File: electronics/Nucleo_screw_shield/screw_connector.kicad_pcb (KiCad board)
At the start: 2 copper layers, 91 x 101.3 mm, 360 parts, among them J1 Conn_01x03, J10 Conn_01x06, J11 Conn_01x10, J12 Conn_01x08, J13 Conn_01x03, J14 Conn_01x03, J15 Conn_01x03, J16 Conn_01x03, J17 Conn_01x03, J18 Conn_01x02, J19 Conn_01x03, J2 Conn_02x19_Odd_Even, J20 Conn_01x03, J21 Conn_01x03, J22 Conn_01x03, J23 Conn_01x03, J3 Conn_01x08, J4 Conn_01x06, J5 Conn_01x10, J6 Conn_01x08, J7 Conn_02x19_Odd_Even, J8 Conn_01x03, J9 Conn_01x08

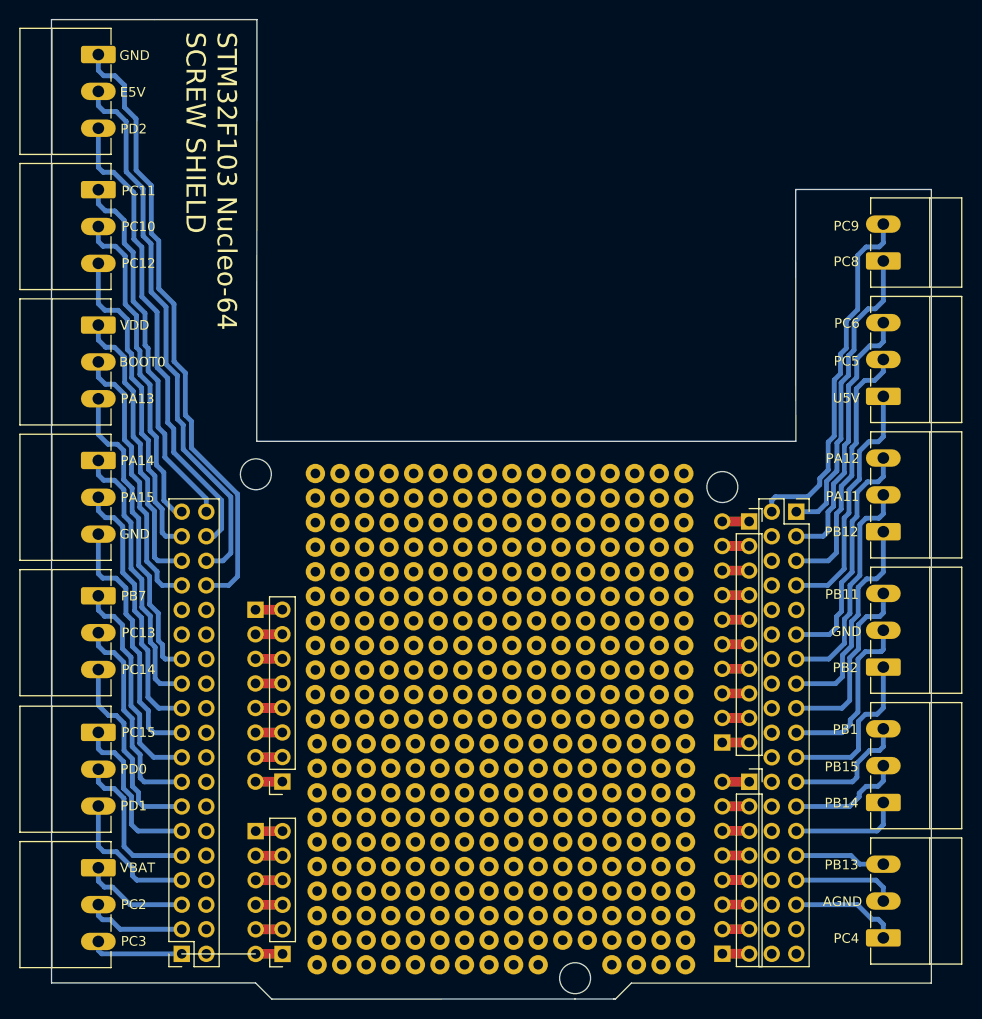
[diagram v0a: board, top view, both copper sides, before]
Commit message: Reorganize CAD files
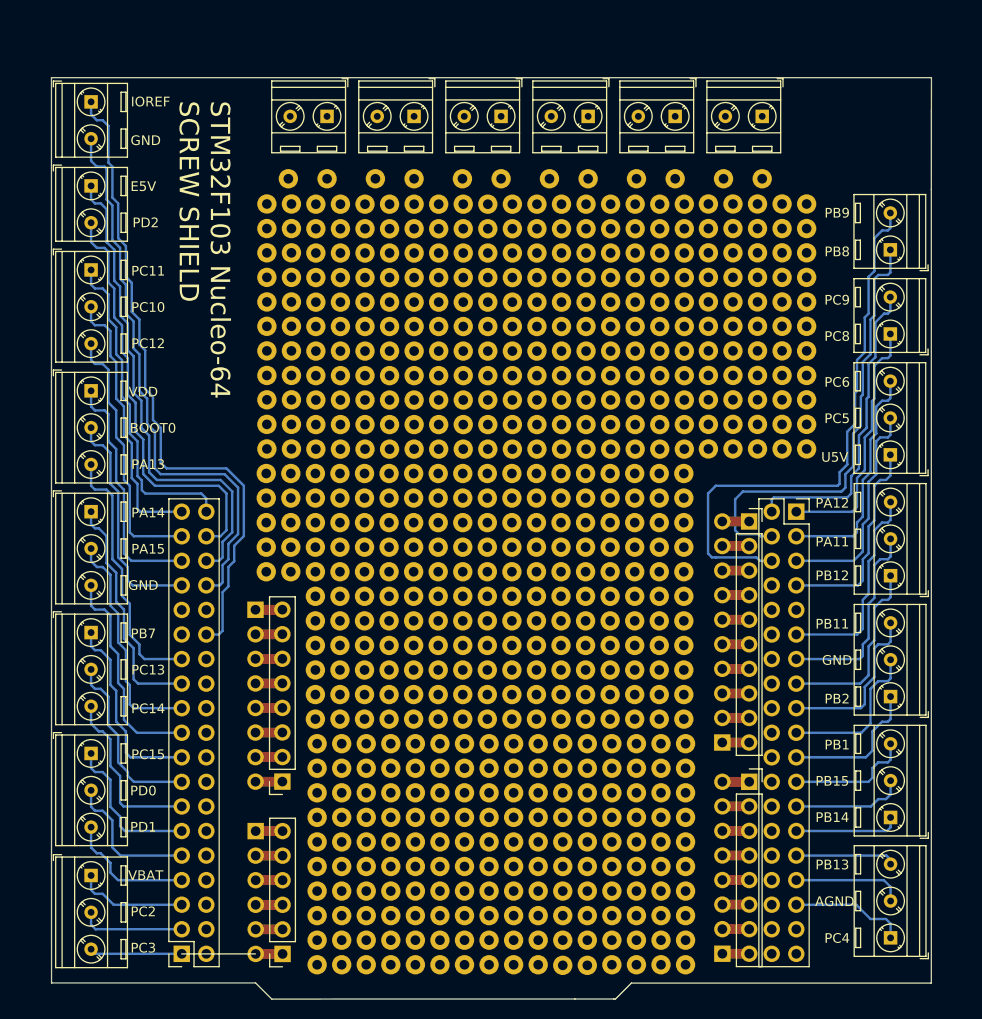
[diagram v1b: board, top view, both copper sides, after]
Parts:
- removed the REF** at (164.7, 146.1)
- removed the REF** at (179.9, 95.3)
- removed the REF** at (131.6, 94.0)
- added J24: Conn_01x02, TerminalBlock_MetzConnect:TerminalBlock_MetzConnect_Type086_RT03402HBLC_1x02_P3.81mm_Horizontal, F.Cu at (114.6, 64.2)
- added J25: Conn_01x02, TerminalBlock_MetzConnect:TerminalBlock_MetzConnect_Type086_RT03402HBLC_1x02_P3.81mm_Horizontal, F.Cu at (197.2, 70.8)
- added J26: Conn_01x02, TerminalBlock_MetzConnect:TerminalBlock_MetzConnect_Type086_RT03402HBLC_1x02_P3.81mm_Horizontal, F.Cu at (184.0, 57.0)
- added J27: Conn_01x02, TerminalBlock_MetzConnect:TerminalBlock_MetzConnect_Type086_RT03402HBLC_1x02_P3.81mm_Horizontal, F.Cu at (139.0, 57.0)
- added J28: Conn_01x02, TerminalBlock_MetzConnect:TerminalBlock_MetzConnect_Type086_RT03402HBLC_1x02_P3.81mm_Horizontal, F.Cu at (175.0, 57.0)
- added J29: Conn_01x02, TerminalBlock_MetzConnect:TerminalBlock_MetzConnect_Type086_RT03402HBLC_1x02_P3.81mm_Horizontal, F.Cu at (148.0, 57.0)
- added J30: Conn_01x02, TerminalBlock_MetzConnect:TerminalBlock_MetzConnect_Type086_RT03402HBLC_1x02_P3.81mm_Horizontal, F.Cu at (166.0, 57.0)
- added J31: Conn_01x02, TerminalBlock_MetzConnect:TerminalBlock_MetzConnect_Type086_RT03402HBLC_1x02_P3.81mm_Horizontal, F.Cu at (157.0, 57.0)
- added REF**: hole 1mm, Connector_PinHeader_2.54mm:hole 1mm, F.Cu at (186.1, 66.1)
- added REF**: hole 1mm, Connector_PinHeader_2.54mm:hole 1mm, F.Cu at (181.0, 66.1)
- added REF**: hole 1mm, Connector_PinHeader_2.54mm:hole 1mm, F.Cu at (137.8, 68.7)
- added REF**: hole 1mm, Connector_PinHeader_2.54mm:hole 1mm, F.Cu at (175.9, 66.1)
- added REF**: hole 1mm, Connector_PinHeader_2.54mm:hole 1mm, F.Cu at (163.2, 66.1)
- added REF**: hole 1mm, Connector_PinHeader_2.54mm:hole 1mm, F.Cu at (160.7, 66.1)
- added REF**: hole 1mm, Connector_PinHeader_2.54mm:hole 1mm, F.Cu at (158.2, 68.7)
- added REF**: hole 1mm, Connector_PinHeader_2.54mm:hole 1mm, F.Cu at (145.5, 68.7)
- added REF**: hole 1mm, Connector_PinHeader_2.54mm:hole 1mm, F.Cu at (150.5, 68.7)
- added REF**: hole 1mm, Connector_PinHeader_2.54mm:hole 1mm, F.Cu at (155.6, 68.7)
- added REF**: hole 1mm, Connector_PinHeader_2.54mm:hole 1mm, F.Cu at (142.9, 66.1)
- added REF**: hole 1mm, Connector_PinHeader_2.54mm:hole 1mm, F.Cu at (148.0, 66.1)
- added REF**: hole 1mm, Connector_PinHeader_2.54mm:hole 1mm, F.Cu at (178.4, 88.9)
- added REF**: hole 1mm, Connector_PinHeader_2.54mm:hole 1mm, F.Cu at (140.4, 68.7)
- added REF**: hole 1mm, Connector_PinHeader_2.54mm:hole 1mm, F.Cu at (155.6, 66.1)
- added REF**: hole 1mm, Connector_PinHeader_2.54mm:hole 1mm, F.Cu at (142.9, 68.7)
- added REF**: hole 1mm, Connector_PinHeader_2.54mm:hole 1mm, F.Cu at (173.4, 68.7)
- added REF**: hole 1mm, Connector_PinHeader_2.54mm:hole 1mm, F.Cu at (170.9, 66.1)
- added REF**: hole 1mm, Connector_PinHeader_2.54mm:hole 1mm, F.Cu at (168.3, 66.1)
- added REF**: hole 1mm, Connector_PinHeader_2.54mm:hole 1mm, F.Cu at (158.2, 66.1)
- added REF**: hole 1mm, Connector_PinHeader_2.54mm:hole 1mm, F.Cu at (170.9, 68.7)
- added REF**: hole 1mm, Connector_PinHeader_2.54mm:hole 1mm, F.Cu at (163.2, 68.7)
- added REF**: hole 1mm, Connector_PinHeader_2.54mm:hole 1mm, F.Cu at (165.8, 68.7)
- added REF**: hole 1mm, Connector_PinHeader_2.54mm:hole 1mm, F.Cu at (186.1, 91.4)
- added REF**: hole 1mm, Connector_PinHeader_2.54mm:hole 1mm, F.Cu at (165.9, 144.8)
- added REF**: hole 1mm, Connector_PinHeader_2.54mm:hole 1mm, F.Cu at (163.4, 144.8)
- added REF**: hole 1mm, Connector_PinHeader_2.54mm:hole 1mm, F.Cu at (148.0, 76.3)
- added REF**: hole 1mm, Connector_PinHeader_2.54mm:hole 1mm, F.Cu at (145.5, 76.3)
- added REF**: hole 1mm, Connector_PinHeader_2.54mm:hole 1mm, F.Cu at (150.5, 76.3)
- added REF**: hole 1mm, Connector_PinHeader_2.54mm:hole 1mm, F.Cu at (153.1, 76.3)
- added REF**: hole 1mm, Connector_PinHeader_2.54mm:hole 1mm, F.Cu at (140.4, 76.3)
- added REF**: hole 1mm, Connector_PinHeader_2.54mm:hole 1mm, F.Cu at (142.9, 76.3)
- added REF**: hole 1mm, Connector_PinHeader_2.54mm:hole 1mm, F.Cu at (137.8, 76.3)
- added REF**: hole 1mm, Connector_PinHeader_2.54mm:hole 1mm, F.Cu at (153.1, 71.2)
- added REF**: hole 1mm, Connector_PinHeader_2.54mm:hole 1mm, F.Cu at (178.4, 91.4)
- added REF**: hole 1mm, Connector_PinHeader_2.54mm:hole 1mm, F.Cu at (145.5, 71.2)
- added REF**: hole 1mm, Connector_PinHeader_2.54mm:hole 1mm, F.Cu at (137.8, 71.2)
- added REF**: hole 1mm, Connector_PinHeader_2.54mm:hole 1mm, F.Cu at (173.4, 71.2)
- added REF**: hole 1mm, Connector_PinHeader_2.54mm:hole 1mm, F.Cu at (140.4, 71.2)
- added REF**: hole 1mm, Connector_PinHeader_2.54mm:hole 1mm, F.Cu at (158.2, 71.2)
- added REF**: hole 1mm, Connector_PinHeader_2.54mm:hole 1mm, F.Cu at (170.9, 73.7)
- added REF**: hole 1mm, Connector_PinHeader_2.54mm:hole 1mm, F.Cu at (142.9, 73.7)
- added REF**: hole 1mm, Connector_PinHeader_2.54mm:hole 1mm, F.Cu at (168.3, 71.2)
- added REF**: hole 1mm, Connector_PinHeader_2.54mm:hole 1mm, F.Cu at (170.9, 71.2)
- added REF**: hole 1mm, Connector_PinHeader_2.54mm:hole 1mm, F.Cu at (173.4, 73.7)
- added REF**: hole 1mm, Connector_PinHeader_2.54mm:hole 1mm, F.Cu at (188.6, 88.9)
- added REF**: hole 1mm, Connector_PinHeader_2.54mm:hole 1mm, F.Cu at (155.6, 73.7)
- added REF**: hole 1mm, Connector_PinHeader_2.54mm:hole 1mm, F.Cu at (155.6, 71.2)
- added REF**: hole 1mm, Connector_PinHeader_2.54mm:hole 1mm, F.Cu at (140.4, 73.7)
- added REF**: hole 1mm, Connector_PinHeader_2.54mm:hole 1mm, F.Cu at (148.0, 71.2)
- added REF**: hole 1mm, Connector_PinHeader_2.54mm:hole 1mm, F.Cu at (142.9, 71.2)
- added REF**: hole 1mm, Connector_PinHeader_2.54mm:hole 1mm, F.Cu at (150.5, 73.7)
- added REF**: hole 1mm, Connector_PinHeader_2.54mm:hole 1mm, F.Cu at (163.2, 73.7)
- added REF**: hole 1mm, Connector_PinHeader_2.54mm:hole 1mm, F.Cu at (160.7, 76.3)
- added REF**: hole 1mm, Connector_PinHeader_2.54mm:hole 1mm, F.Cu at (163.2, 76.3)
- added REF**: hole 1mm, Connector_PinHeader_2.54mm:hole 1mm, F.Cu at (155.6, 76.3)
- added REF**: hole 1mm, Connector_PinHeader_2.54mm:hole 1mm, F.Cu at (181.0, 88.9)
- added REF**: hole 1mm, Connector_PinHeader_2.54mm:hole 1mm, F.Cu at (158.2, 76.3)
- added REF**: hole 1mm, Connector_PinHeader_2.54mm:hole 1mm, F.Cu at (165.8, 73.7)
- added REF**: hole 1mm, Connector_PinHeader_2.54mm:hole 1mm, F.Cu at (158.2, 73.7)
- added REF**: hole 1mm, Connector_PinHeader_2.54mm:hole 1mm, F.Cu at (153.1, 73.7)
- added REF**: hole 1mm, Connector_PinHeader_2.54mm:hole 1mm, F.Cu at (145.5, 73.7)
- added REF**: hole 1mm, Connector_PinHeader_2.54mm:hole 1mm, F.Cu at (148.0, 73.7)
- added REF**: hole 1mm, Connector_PinHeader_2.54mm:hole 1mm, F.Cu at (160.7, 73.7)
- added REF**: hole 1mm, Connector_PinHeader_2.54mm:hole 1mm, F.Cu at (173.4, 76.3)
- added REF**: hole 1mm, Connector_PinHeader_2.54mm:hole 1mm, F.Cu at (168.3, 73.7)
- added REF**: hole 1mm, Connector_PinHeader_2.54mm:hole 1mm, F.Cu at (137.8, 73.7)
- added REF**: hole 1mm, Connector_PinHeader_2.54mm:hole 1mm, F.Cu at (183.5, 91.4)
- added REF**: hole 1mm, Connector_PinHeader_2.54mm:hole 1mm, F.Cu at (168.3, 76.3)
- added REF**: hole 1mm, Connector_PinHeader_2.54mm:hole 1mm, F.Cu at (170.9, 76.3)
- added REF**: hole 1mm, Connector_PinHeader_2.54mm:hole 1mm, F.Cu at (175.9, 73.7)
- added REF**: hole 1mm, Connector_PinHeader_2.54mm:hole 1mm, F.Cu at (165.8, 76.3)
- added REF**: hole 1mm, Connector_PinHeader_2.54mm:hole 1mm, F.Cu at (150.5, 71.2)
- added REF**: hole 1mm, Connector_PinHeader_2.54mm:hole 1mm, F.Cu at (160.7, 71.2)
- added REF**: hole 1mm, Connector_PinHeader_2.54mm:hole 1mm, F.Cu at (165.8, 71.2)
- added REF**: hole 1mm, Connector_PinHeader_2.54mm:hole 1mm, F.Cu at (163.2, 71.2)
- added REF**: hole 1mm, Connector_PinHeader_2.54mm:hole 1mm, F.Cu at (175.9, 71.2)
- added REF**: hole 1mm, Connector_PinHeader_2.54mm:hole 1mm, F.Cu at (175.9, 76.3)
- added REF**: hole 1mm, Connector_PinHeader_2.54mm:hole 1mm, F.Cu at (181.0, 91.4)
- added REF**: hole 1mm, Connector_PinHeader_2.54mm:hole 1mm, F.Cu at (148.0, 83.9)
- added REF**: hole 1mm, Connector_PinHeader_2.54mm:hole 1mm, F.Cu at (145.5, 83.9)
- added REF**: hole 1mm, Connector_PinHeader_2.54mm:hole 1mm, F.Cu at (150.5, 83.9)
- added REF**: hole 1mm, Connector_PinHeader_2.54mm:hole 1mm, F.Cu at (153.1, 83.9)
- added REF**: hole 1mm, Connector_PinHeader_2.54mm:hole 1mm, F.Cu at (140.4, 83.9)
- added REF**: hole 1mm, Connector_PinHeader_2.54mm:hole 1mm, F.Cu at (142.9, 83.9)
- added REF**: hole 1mm, Connector_PinHeader_2.54mm:hole 1mm, F.Cu at (137.8, 83.9)
- added REF**: hole 1mm, Connector_PinHeader_2.54mm:hole 1mm, F.Cu at (153.1, 78.8)
- added REF**: hole 1mm, Connector_PinHeader_2.54mm:hole 1mm, F.Cu at (145.5, 78.8)
- added REF**: hole 1mm, Connector_PinHeader_2.54mm:hole 1mm, F.Cu at (137.8, 78.8)
- added REF**: hole 1mm, Connector_PinHeader_2.54mm:hole 1mm, F.Cu at (183.5, 86.4)
- added REF**: hole 1mm, Connector_PinHeader_2.54mm:hole 1mm, F.Cu at (173.4, 78.8)
- added REF**: hole 1mm, Connector_PinHeader_2.54mm:hole 1mm, F.Cu at (140.4, 78.8)
- added REF**: hole 1mm, Connector_PinHeader_2.54mm:hole 1mm, F.Cu at (158.2, 78.8)
- added REF**: hole 1mm, Connector_PinHeader_2.54mm:hole 1mm, F.Cu at (170.9, 81.3)
- added REF**: hole 1mm, Connector_PinHeader_2.54mm:hole 1mm, F.Cu at (142.9, 81.3)
- added REF**: hole 1mm, Connector_PinHeader_2.54mm:hole 1mm, F.Cu at (168.3, 78.8)
- added REF**: hole 1mm, Connector_PinHeader_2.54mm:hole 1mm, F.Cu at (170.9, 78.8)
- added REF**: hole 1mm, Connector_PinHeader_2.54mm:hole 1mm, F.Cu at (173.4, 81.3)
- added REF**: hole 1mm, Connector_PinHeader_2.54mm:hole 1mm, F.Cu at (155.6, 81.3)
- added REF**: hole 1mm, Connector_PinHeader_2.54mm:hole 1mm, F.Cu at (155.6, 78.8)
- added REF**: hole 1mm, Connector_PinHeader_2.54mm:hole 1mm, F.Cu at (183.5, 88.9)
- added REF**: hole 1mm, Connector_PinHeader_2.54mm:hole 1mm, F.Cu at (140.4, 81.3)
- added REF**: hole 1mm, Connector_PinHeader_2.54mm:hole 1mm, F.Cu at (148.0, 78.8)
- added REF**: hole 1mm, Connector_PinHeader_2.54mm:hole 1mm, F.Cu at (142.9, 78.8)
- added REF**: hole 1mm, Connector_PinHeader_2.54mm:hole 1mm, F.Cu at (150.5, 81.3)
- added REF**: hole 1mm, Connector_PinHeader_2.54mm:hole 1mm, F.Cu at (163.2, 81.3)
- added REF**: hole 1mm, Connector_PinHeader_2.54mm:hole 1mm, F.Cu at (160.7, 83.9)
- added REF**: hole 1mm, Connector_PinHeader_2.54mm:hole 1mm, F.Cu at (163.2, 83.9)
- added REF**: hole 1mm, Connector_PinHeader_2.54mm:hole 1mm, F.Cu at (155.6, 83.9)
- added REF**: hole 1mm, Connector_PinHeader_2.54mm:hole 1mm, F.Cu at (158.2, 83.9)
- added REF**: hole 1mm, Connector_PinHeader_2.54mm:hole 1mm, F.Cu at (165.8, 81.3)
- added REF**: hole 1mm, Connector_PinHeader_2.54mm:hole 1mm, F.Cu at (178.4, 66.1)
- added REF**: hole 1mm, Connector_PinHeader_2.54mm:hole 1mm, F.Cu at (186.1, 88.9)
- added REF**: hole 1mm, Connector_PinHeader_2.54mm:hole 1mm, F.Cu at (158.2, 81.3)
- added REF**: hole 1mm, Connector_PinHeader_2.54mm:hole 1mm, F.Cu at (153.1, 81.3)
- added REF**: hole 1mm, Connector_PinHeader_2.54mm:hole 1mm, F.Cu at (145.5, 81.3)
- added REF**: hole 1mm, Connector_PinHeader_2.54mm:hole 1mm, F.Cu at (148.0, 81.3)
- added REF**: hole 1mm, Connector_PinHeader_2.54mm:hole 1mm, F.Cu at (160.7, 81.3)
- added REF**: hole 1mm, Connector_PinHeader_2.54mm:hole 1mm, F.Cu at (173.4, 83.9)
- added REF**: hole 1mm, Connector_PinHeader_2.54mm:hole 1mm, F.Cu at (168.3, 81.3)
- added REF**: hole 1mm, Connector_PinHeader_2.54mm:hole 1mm, F.Cu at (137.8, 81.3)
- added REF**: hole 1mm, Connector_PinHeader_2.54mm:hole 1mm, F.Cu at (168.3, 83.9)
- added REF**: hole 1mm, Connector_PinHeader_2.54mm:hole 1mm, F.Cu at (170.9, 83.9)
- added REF**: hole 1mm, Connector_PinHeader_2.54mm:hole 1mm, F.Cu at (181.0, 86.4)
- added REF**: hole 1mm, Connector_PinHeader_2.54mm:hole 1mm, F.Cu at (175.9, 81.3)
- added REF**: hole 1mm, Connector_PinHeader_2.54mm:hole 1mm, F.Cu at (165.8, 83.9)
- added REF**: hole 1mm, Connector_PinHeader_2.54mm:hole 1mm, F.Cu at (150.5, 78.8)
- added REF**: hole 1mm, Connector_PinHeader_2.54mm:hole 1mm, F.Cu at (160.7, 78.8)
- added REF**: hole 1mm, Connector_PinHeader_2.54mm:hole 1mm, F.Cu at (165.8, 78.8)
- added REF**: hole 1mm, Connector_PinHeader_2.54mm:hole 1mm, F.Cu at (163.2, 78.8)
- added REF**: hole 1mm, Connector_PinHeader_2.54mm:hole 1mm, F.Cu at (175.9, 78.8)
- added REF**: hole 1mm, Connector_PinHeader_2.54mm:hole 1mm, F.Cu at (175.9, 83.9)
- added REF**: hole 1mm, Connector_PinHeader_2.54mm:hole 1mm, F.Cu at (148.0, 91.5)
- added REF**: hole 1mm, Connector_PinHeader_2.54mm:hole 1mm, F.Cu at (145.5, 91.5)
- added REF**: hole 1mm, Connector_PinHeader_2.54mm:hole 1mm, F.Cu at (186.1, 86.4)
- added REF**: hole 1mm, Connector_PinHeader_2.54mm:hole 1mm, F.Cu at (150.5, 91.5)
- added REF**: hole 1mm, Connector_PinHeader_2.54mm:hole 1mm, F.Cu at (153.1, 91.5)
- added REF**: hole 1mm, Connector_PinHeader_2.54mm:hole 1mm, F.Cu at (140.4, 91.5)
- added REF**: hole 1mm, Connector_PinHeader_2.54mm:hole 1mm, F.Cu at (142.9, 91.5)
- added REF**: hole 1mm, Connector_PinHeader_2.54mm:hole 1mm, F.Cu at (137.8, 91.5)
- added REF**: hole 1mm, Connector_PinHeader_2.54mm:hole 1mm, F.Cu at (153.1, 86.4)
- added REF**: hole 1mm, Connector_PinHeader_2.54mm:hole 1mm, F.Cu at (145.5, 86.4)
- added REF**: hole 1mm, Connector_PinHeader_2.54mm:hole 1mm, F.Cu at (137.8, 86.4)
- added REF**: hole 1mm, Connector_PinHeader_2.54mm:hole 1mm, F.Cu at (173.4, 86.4)
- added REF**: hole 1mm, Connector_PinHeader_2.54mm:hole 1mm, F.Cu at (140.4, 86.4)
- added REF**: hole 1mm, Connector_PinHeader_2.54mm:hole 1mm, F.Cu at (186.1, 78.8)
- added REF**: hole 1mm, Connector_PinHeader_2.54mm:hole 1mm, F.Cu at (158.2, 86.4)
- added REF**: hole 1mm, Connector_PinHeader_2.54mm:hole 1mm, F.Cu at (170.9, 88.9)
- added REF**: hole 1mm, Connector_PinHeader_2.54mm:hole 1mm, F.Cu at (142.9, 88.9)
- added REF**: hole 1mm, Connector_PinHeader_2.54mm:hole 1mm, F.Cu at (168.3, 86.4)
- added REF**: hole 1mm, Connector_PinHeader_2.54mm:hole 1mm, F.Cu at (170.9, 86.4)
- added REF**: hole 1mm, Connector_PinHeader_2.54mm:hole 1mm, F.Cu at (173.4, 88.9)
- added REF**: hole 1mm, Connector_PinHeader_2.54mm:hole 1mm, F.Cu at (155.6, 88.9)
- added REF**: hole 1mm, Connector_PinHeader_2.54mm:hole 1mm, F.Cu at (155.6, 86.4)
- added REF**: hole 1mm, Connector_PinHeader_2.54mm:hole 1mm, F.Cu at (140.4, 88.9)
- added REF**: hole 1mm, Connector_PinHeader_2.54mm:hole 1mm, F.Cu at (148.0, 86.4)
- added REF**: hole 1mm, Connector_PinHeader_2.54mm:hole 1mm, F.Cu at (186.1, 81.3)
- added REF**: hole 1mm, Connector_PinHeader_2.54mm:hole 1mm, F.Cu at (142.9, 86.4)
- added REF**: hole 1mm, Connector_PinHeader_2.54mm:hole 1mm, F.Cu at (150.5, 88.9)
- added REF**: hole 1mm, Connector_PinHeader_2.54mm:hole 1mm, F.Cu at (163.2, 88.9)
- added REF**: hole 1mm, Connector_PinHeader_2.54mm:hole 1mm, F.Cu at (160.7, 91.5)
- added REF**: hole 1mm, Connector_PinHeader_2.54mm:hole 1mm, F.Cu at (163.2, 91.5)
- added REF**: hole 1mm, Connector_PinHeader_2.54mm:hole 1mm, F.Cu at (155.6, 91.5)
- added REF**: hole 1mm, Connector_PinHeader_2.54mm:hole 1mm, F.Cu at (158.2, 91.5)
- added REF**: hole 1mm, Connector_PinHeader_2.54mm:hole 1mm, F.Cu at (165.8, 88.9)
- added REF**: hole 1mm, Connector_PinHeader_2.54mm:hole 1mm, F.Cu at (158.2, 88.9)
- added REF**: hole 1mm, Connector_PinHeader_2.54mm:hole 1mm, F.Cu at (153.1, 88.9)
- added REF**: hole 1mm, Connector_PinHeader_2.54mm:hole 1mm, F.Cu at (181.0, 78.8)
- added REF**: hole 1mm, Connector_PinHeader_2.54mm:hole 1mm, F.Cu at (145.5, 88.9)
- added REF**: hole 1mm, Connector_PinHeader_2.54mm:hole 1mm, F.Cu at (148.0, 88.9)
- added REF**: hole 1mm, Connector_PinHeader_2.54mm:hole 1mm, F.Cu at (160.7, 88.9)
- added REF**: hole 1mm, Connector_PinHeader_2.54mm:hole 1mm, F.Cu at (173.4, 91.5)
- added REF**: hole 1mm, Connector_PinHeader_2.54mm:hole 1mm, F.Cu at (168.3, 88.9)
- added REF**: hole 1mm, Connector_PinHeader_2.54mm:hole 1mm, F.Cu at (137.8, 88.9)
- added REF**: hole 1mm, Connector_PinHeader_2.54mm:hole 1mm, F.Cu at (168.3, 91.5)
- added REF**: hole 1mm, Connector_PinHeader_2.54mm:hole 1mm, F.Cu at (170.9, 91.5)
- added REF**: hole 1mm, Connector_PinHeader_2.54mm:hole 1mm, F.Cu at (175.9, 88.9)
- added REF**: hole 1mm, Connector_PinHeader_2.54mm:hole 1mm, F.Cu at (165.8, 91.5)
- added REF**: hole 1mm, Connector_PinHeader_2.54mm:hole 1mm, F.Cu at (183.5, 78.8)
- added REF**: hole 1mm, Connector_PinHeader_2.54mm:hole 1mm, F.Cu at (150.5, 86.4)
- added REF**: hole 1mm, Connector_PinHeader_2.54mm:hole 1mm, F.Cu at (160.7, 86.4)
- added REF**: hole 1mm, Connector_PinHeader_2.54mm:hole 1mm, F.Cu at (165.8, 86.4)
- added REF**: hole 1mm, Connector_PinHeader_2.54mm:hole 1mm, F.Cu at (163.2, 86.4)
- added REF**: hole 1mm, Connector_PinHeader_2.54mm:hole 1mm, F.Cu at (175.9, 86.4)
- added REF**: hole 1mm, Connector_PinHeader_2.54mm:hole 1mm, F.Cu at (175.9, 91.5)
- added REF**: hole 1mm, Connector_PinHeader_2.54mm:hole 1mm, F.Cu at (135.0, 63.5)
- added REF**: hole 1mm, Connector_PinHeader_2.54mm:hole 1mm, F.Cu at (139.0, 63.5)
- added REF**: hole 1mm, Connector_PinHeader_2.54mm:hole 1mm, F.Cu at (144.0, 63.5)
- added REF**: hole 1mm, Connector_PinHeader_2.54mm:hole 1mm, F.Cu at (148.0, 63.5)
- added REF**: hole 1mm, Connector_PinHeader_2.54mm:hole 1mm, F.Cu at (183.5, 81.3)
- added REF**: hole 1mm, Connector_PinHeader_2.54mm:hole 1mm, F.Cu at (153.0, 63.5)
- added REF**: hole 1mm, Connector_PinHeader_2.54mm:hole 1mm, F.Cu at (157.0, 63.5)
- added REF**: hole 1mm, Connector_PinHeader_2.54mm:hole 1mm, F.Cu at (162.0, 63.5)
- added REF**: hole 1mm, Connector_PinHeader_2.54mm:hole 1mm, F.Cu at (166.0, 63.5)
- added REF**: hole 1mm, Connector_PinHeader_2.54mm:hole 1mm, F.Cu at (171.0, 63.5)
- added REF**: hole 1mm, Connector_PinHeader_2.54mm:hole 1mm, F.Cu at (175.0, 63.5)
- added REF**: hole 1mm, Connector_PinHeader_2.54mm:hole 1mm, F.Cu at (180.0, 63.5)
- added REF**: hole 1mm, Connector_PinHeader_2.54mm:hole 1mm, F.Cu at (184.0, 63.5)
- added REF**: hole 1mm, Connector_PinHeader_2.54mm:hole 1mm, F.Cu at (178.4, 78.8)
- added REF**: hole 1mm, Connector_PinHeader_2.54mm:hole 1mm, F.Cu at (183.5, 83.8)
- added REF**: hole 1mm, Connector_PinHeader_2.54mm:hole 1mm, F.Cu at (181.0, 68.7)
- added REF**: hole 1mm, Connector_PinHeader_2.54mm:hole 1mm, F.Cu at (188.6, 83.8)
- added REF**: hole 1mm, Connector_PinHeader_2.54mm:hole 1mm, F.Cu at (188.6, 81.3)
- added REF**: hole 1mm, Connector_PinHeader_2.54mm:hole 1mm, F.Cu at (181.0, 81.3)
- added REF**: hole 1mm, Connector_PinHeader_2.54mm:hole 1mm, F.Cu at (178.4, 83.8)
- added REF**: hole 1mm, Connector_PinHeader_2.54mm:hole 1mm, F.Cu at (181.0, 83.8)
- added REF**: hole 1mm, Connector_PinHeader_2.54mm:hole 1mm, F.Cu at (188.6, 78.8)
- added REF**: hole 1mm, Connector_PinHeader_2.54mm:hole 1mm, F.Cu at (186.1, 71.2)
- added REF**: hole 1mm, Connector_PinHeader_2.54mm:hole 1mm, F.Cu at (178.4, 71.2)
- added REF**: hole 1mm, Connector_PinHeader_2.54mm:hole 1mm, F.Cu at (186.1, 76.2)
- added REF**: hole 1mm, Connector_PinHeader_2.54mm:hole 1mm, F.Cu at (181.0, 73.7)
- added REF**: hole 1mm, Connector_PinHeader_2.54mm:hole 1mm, F.Cu at (188.6, 68.7)
- added REF**: hole 1mm, Connector_PinHeader_2.54mm:hole 1mm, F.Cu at (188.6, 73.7)
- added REF**: hole 1mm, Connector_PinHeader_2.54mm:hole 1mm, F.Cu at (183.5, 76.2)
- added REF**: hole 1mm, Connector_PinHeader_2.54mm:hole 1mm, F.Cu at (188.6, 71.2)
- added REF**: hole 1mm, Connector_PinHeader_2.54mm:hole 1mm, F.Cu at (178.4, 76.2)
- added REF**: hole 1mm, Connector_PinHeader_2.54mm:hole 1mm, F.Cu at (181.0, 76.2)
- added REF**: hole 1mm, Connector_PinHeader_2.54mm:hole 1mm, F.Cu at (188.6, 76.2)
- added REF**: hole 1mm, Connector_PinHeader_2.54mm:hole 1mm, F.Cu at (186.1, 73.7)
- added REF**: hole 1mm, Connector_PinHeader_2.54mm:hole 1mm, F.Cu at (183.5, 71.2)
- added REF**: hole 1mm, Connector_PinHeader_2.54mm:hole 1mm, F.Cu at (181.0, 71.2)
- added REF**: hole 1mm, Connector_PinHeader_2.54mm:hole 1mm, F.Cu at (183.5, 73.7)
- added REF**: hole 1mm, Connector_PinHeader_2.54mm:hole 1mm, F.Cu at (188.6, 66.1)
- added REF**: hole 1mm, Connector_PinHeader_2.54mm:hole 1mm, F.Cu at (178.4, 73.7)
- added REF**: hole 1mm, Connector_PinHeader_2.54mm:hole 1mm, F.Cu at (188.6, 86.4)
- added REF**: hole 1mm, Connector_PinHeader_2.54mm:hole 1mm, F.Cu at (188.6, 91.4)
- added REF**: hole 1mm, Connector_PinHeader_2.54mm:hole 1mm, F.Cu at (178.4, 86.4)
- added REF**: hole 1mm, Connector_PinHeader_2.54mm:hole 1mm, F.Cu at (186.1, 83.8)
- added REF**: hole 1mm, Connector_PinHeader_2.54mm:hole 1mm, F.Cu at (178.4, 81.3)
- added REF**: hole 1mm, Connector_PinHeader_2.54mm:hole 1mm, F.Cu at (132.7, 101.6)
- added REF**: hole 1mm, Connector_PinHeader_2.54mm:hole 1mm, F.Cu at (132.7, 104.1)
- added REF**: hole 1mm, Connector_PinHeader_2.54mm:hole 1mm, F.Cu at (132.7, 99.1)
- added REF**: hole 1mm, Connector_PinHeader_2.54mm:hole 1mm, F.Cu at (132.7, 94.0)
- added REF**: hole 1mm, Connector_PinHeader_2.54mm:hole 1mm, F.Cu at (186.1, 68.7)
- added REF**: hole 1mm, Connector_PinHeader_2.54mm:hole 1mm, F.Cu at (132.7, 96.5)
- added REF**: hole 1mm, Connector_PinHeader_2.54mm:hole 1mm, F.Cu at (135.3, 101.6)
- added REF**: hole 1mm, Connector_PinHeader_2.54mm:hole 1mm, F.Cu at (135.3, 104.1)
- added REF**: hole 1mm, Connector_PinHeader_2.54mm:hole 1mm, F.Cu at (135.3, 99.1)
- added REF**: hole 1mm, Connector_PinHeader_2.54mm:hole 1mm, F.Cu at (135.3, 94.0)
- added REF**: hole 1mm, Connector_PinHeader_2.54mm:hole 1mm, F.Cu at (135.3, 96.5)
- added REF**: hole 1mm, Connector_PinHeader_2.54mm:hole 1mm, F.Cu at (135.3, 66.1)
- added REF**: hole 1mm, Connector_PinHeader_2.54mm:hole 1mm, F.Cu at (132.8, 66.1)
- added REF**: hole 1mm, Connector_PinHeader_2.54mm:hole 1mm, F.Cu at (132.8, 68.7)
- added REF**: hole 1mm, Connector_PinHeader_2.54mm:hole 1mm, F.Cu at (135.3, 68.7)
- added REF**: hole 1mm, Connector_PinHeader_2.54mm:hole 1mm, F.Cu at (183.5, 66.1)
- added REF**: hole 1mm, Connector_PinHeader_2.54mm:hole 1mm, F.Cu at (132.8, 88.9)
- added REF**: hole 1mm, Connector_PinHeader_2.54mm:hole 1mm, F.Cu at (132.8, 91.4)
- added REF**: hole 1mm, Connector_PinHeader_2.54mm:hole 1mm, F.Cu at (135.3, 88.9)
- added REF**: hole 1mm, Connector_PinHeader_2.54mm:hole 1mm, F.Cu at (132.8, 86.4)
- added REF**: hole 1mm, Connector_PinHeader_2.54mm:hole 1mm, F.Cu at (135.3, 86.4)
- added REF**: hole 1mm, Connector_PinHeader_2.54mm:hole 1mm, F.Cu at (135.3, 78.8)
- added REF**: hole 1mm, Connector_PinHeader_2.54mm:hole 1mm, F.Cu at (135.3, 83.8)
- added REF**: hole 1mm, Connector_PinHeader_2.54mm:hole 1mm, F.Cu at (132.8, 78.8)
- added REF**: hole 1mm, Connector_PinHeader_2.54mm:hole 1mm, F.Cu at (132.8, 83.8)
- added REF**: hole 1mm, Connector_PinHeader_2.54mm:hole 1mm, F.Cu at (132.8, 81.3)
- added REF**: hole 1mm, Connector_PinHeader_2.54mm:hole 1mm, F.Cu at (178.4, 68.7)
- added REF**: hole 1mm, Connector_PinHeader_2.54mm:hole 1mm, F.Cu at (135.3, 91.4)
- added REF**: hole 1mm, Connector_PinHeader_2.54mm:hole 1mm, F.Cu at (132.8, 76.2)
- added REF**: hole 1mm, Connector_PinHeader_2.54mm:hole 1mm, F.Cu at (135.3, 71.2)
- added REF**: hole 1mm, Connector_PinHeader_2.54mm:hole 1mm, F.Cu at (132.8, 71.2)
- added REF**: hole 1mm, Connector_PinHeader_2.54mm:hole 1mm, F.Cu at (135.3, 76.2)
- added REF**: hole 1mm, Connector_PinHeader_2.54mm:hole 1mm, F.Cu at (132.8, 73.7)
- added REF**: hole 1mm, Connector_PinHeader_2.54mm:hole 1mm, F.Cu at (135.3, 73.7)
- added REF**: hole 1mm, Connector_PinHeader_2.54mm:hole 1mm, F.Cu at (135.3, 81.3)
- added REF**: hole 1mm, Connector_PinHeader_2.54mm:hole 1mm, F.Cu at (140.4, 66.1)
- added REF**: hole 1mm, Connector_PinHeader_2.54mm:hole 1mm, F.Cu at (173.4, 66.1)
- added REF**: hole 1mm, Connector_PinHeader_2.54mm:hole 1mm, F.Cu at (183.5, 68.7)
- added REF**: hole 1mm, Connector_PinHeader_2.54mm:hole 1mm, F.Cu at (153.1, 66.1)
- added REF**: hole 1mm, Connector_PinHeader_2.54mm:hole 1mm, F.Cu at (137.8, 66.1)
- added REF**: hole 1mm, Connector_PinHeader_2.54mm:hole 1mm, F.Cu at (145.5, 66.1)
- added REF**: hole 1mm, Connector_PinHeader_2.54mm:hole 1mm, F.Cu at (160.7, 68.7)
- added REF**: hole 1mm, Connector_PinHeader_2.54mm:hole 1mm, F.Cu at (165.8, 66.1)
- added REF**: hole 1mm, Connector_PinHeader_2.54mm:hole 1mm, F.Cu at (150.5, 66.1)
- added REF**: hole 1mm, Connector_PinHeader_2.54mm:hole 1mm, F.Cu at (168.3, 68.7)
- added REF**: hole 1mm, Connector_PinHeader_2.54mm:hole 1mm, F.Cu at (175.9, 68.7)
- added REF**: hole 1mm, Connector_PinHeader_2.54mm:hole 1mm, F.Cu at (153.1, 68.7)
- added REF**: hole 1mm, Connector_PinHeader_2.54mm:hole 1mm, F.Cu at (148.0, 68.7)
- J1: value Conn_01x03 -> Conn_01x02; footprint Connector_Phoenix_MC:PhoenixContact_MC_1,5_3-G-3.81_1x03_P3.81mm_Horizontal -> TerminalBlock_MetzConnect:TerminalBlock_MetzConnect_Type086_RT03402HBLC_1x02_P3.81mm_Horizontal
- J13, J14, J15, J16, J17, J19, J20, J21, J22, J23, J8: footprint Connector_Phoenix_MC:PhoenixContact_MC_1,5_3-G-3.81_1x03_P3.81mm_Horizontal -> TerminalBlock_MetzConnect:TerminalBlock_MetzConnect_Type086_RT03403HBLC_1x03_P3.81mm_Horizontal
- J18: footprint Connector_Phoenix_MC:PhoenixContact_MC_1,5_2-G-3.81_1x02_P3.81mm_Horizontal -> TerminalBlock_MetzConnect:TerminalBlock_MetzConnect_Type086_RT03402HBLC_1x02_P3.81mm_Horizontal
- moved J8 8.33 mm to (114.6, 72.9)
- moved J18 7.58 mm to (197.2, 79.5)
- moved J13 6.84 mm to (114.6, 85.4)
- moved J19 6.09 mm to (197.2, 92.0)
- moved J14 5.35 mm to (114.6, 97.9)
- moved J1 4.95 mm to (114.6, 55.5)
- moved J20 4.61 mm to (197.3, 104.5)
- moved J15 3.87 mm to (114.6, 110.4)
- moved J21 3.14 mm to (197.3, 117.0)
- moved J16 2.31 mm to (114.6, 122.9)
- moved J22 1.72 mm to (197.3, 129.5)
- moved J17 1.10 mm to (114.6, 135.5)
- moved J23 0.75 mm to (197.3, 141.9)
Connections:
- J2 pad 28: Net-(J2-Pad28) -> Net-(J1-Pad1)
- J2 pad 32: Net-(J1-Pad1) -> Net-(J1-Pad2)
- J2 pad 34: Net-(J1-Pad2) -> Net-(J2-Pad34)
- J2 pad 36: Net-(J1-Pad3) -> Net-(J2-Pad36)
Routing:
- net Net-(J25-Pad2): track 0.00 -> 57.7 mm
- net Net-(J2-Pad34): track 0.00 -> 50.9 mm
- net Net-(J1-Pad3): track 49.2 -> 0.00 mm
- net Net-(J25-Pad1): track 0.00 -> 46.3 mm
- net Net-(J2-Pad36): track 0.00 -> 44.3 mm
- net Net-(J2-Pad35): track 33.6 -> 27.2 mm
- net Net-(J2-Pad37): track 34.2 -> 28.9 mm
- net Net-(J18-Pad2): track 37.3 -> 32.0 mm
- net Net-(J18-Pad1): track 31.4 -> 26.2 mm
- net Net-(J13-Pad3): track 32.1 -> 27.0 mm
- net Net-(J13-Pad1): track 29.9 -> 25.1 mm
- net Net-(J13-Pad2): track 28.4 -> 23.6 mm
- net Net-(J2-Pad38): track 38.5 -> 33.8 mm
- net Net-(J19-Pad2): track 27.1 -> 22.7 mm
- net Net-(J14-Pad3): track 26.6 -> 22.4 mm
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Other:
- board size 91 x 101.3 mm -> 91 x 95.3 mm
- board text added: "IOREF"
- board text added: "PB8"
- board text added: "PB9"
